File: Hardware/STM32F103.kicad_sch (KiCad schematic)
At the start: 23 parts, among them J12 Conn_01x04_Male, J8 Conn_02x04_Odd_Even, J9 Conn_01x07_Pin, SW3 SW_Push, U5 MCU_STM32F103C8Tx, Y1 8Mhz

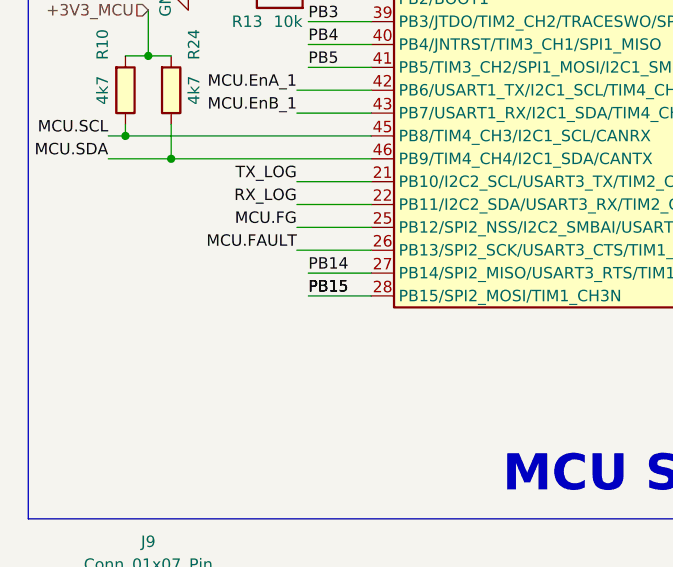
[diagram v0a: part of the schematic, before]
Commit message: Update README
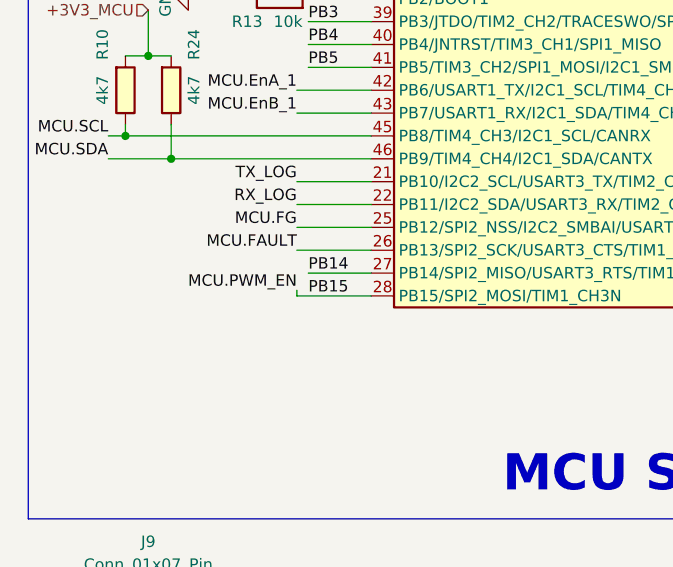
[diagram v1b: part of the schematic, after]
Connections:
- net PB15 renamed MCU.PWM_EN
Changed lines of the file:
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@@
 (kicad_sch (version 20230121) (generator eeschema)
   (paper "A4")
+  (bus_alias "I2C" (members "SCL" "SDA"))
   (bus_alias "SPI" (members "MISO" "MOSI" "SCK" "CS"))
+  (bus_alias "DC_MOTOR" (members "PWM_L1" "PWM_R1" "PWM_L2" "PWM_R2"))
+  (bus_alias "CAN" (members "CANH" "CANL"))
   (bus_alias "En" (members "EnA_1" "EnB_1" "EnA_2" "EnB_2"))
-  (bus_alias "CAN" (members "CANH" "CANL"))
-  (bus_alias "DC_MOTOR" (members "PWM_L1" "PWM_R1" "PWM_L2" "PWM_R2"))
-  (bus_alias "I2C" (members "SCL" "SDA"))
   (junction (at 212.09 124.46) (diameter 0) (color 0 0 0 0)
   )
@@
     (stroke (width 0) (type default))
   )
+  (wire (pts (xy 49.53 122.555) (xy 57.785 122.555))
+    (stroke (width 0) (type default))
+  )
   (bus (pts (xy 266.7 95.25) (xy 266.7 97.79))
     (stroke (width 0) (type default))
@@
     (stroke (width 0) (type default))
   )
-  (wire (pts (xy 50.8 122.555) (xy 57.785 122.555))
-    (stroke (width 0) (type default))
-  )
   (wire (pts (xy 219.71 98.425) (xy 222.885 98.425))
     (stroke (width 0) (type default))
@@
   )
   (wire (pts (xy 113.665 130.175) (xy 113.665 131.445))
+    (stroke (width 0) (type default))
+  )
+  (wire (pts (xy 49.53 121.92) (xy 49.53 122.555))
     (stroke (width 0) (type default))
   )
@@
     (effects (font (size 1.27 1.27)) (justify left bottom))
   )
-  (label "PB15" (at 50.8 122.555 0) (fields_autoplaced)
-    (effects (font (size 1.27 1.27)) (justify left bottom))
+  (label "MCU.PWM_EN" (at 49.53 121.92 180) (fields_autoplaced)
+    (effects (font (size 1.27 1.27)) (justify right bottom))
   )
   (label "PA9" (at 166.37 107.315 0) (fields_autoplaced)
